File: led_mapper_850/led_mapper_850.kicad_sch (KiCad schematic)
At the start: 1082 parts, among them J1 Conn_02x12_Top_Bottom

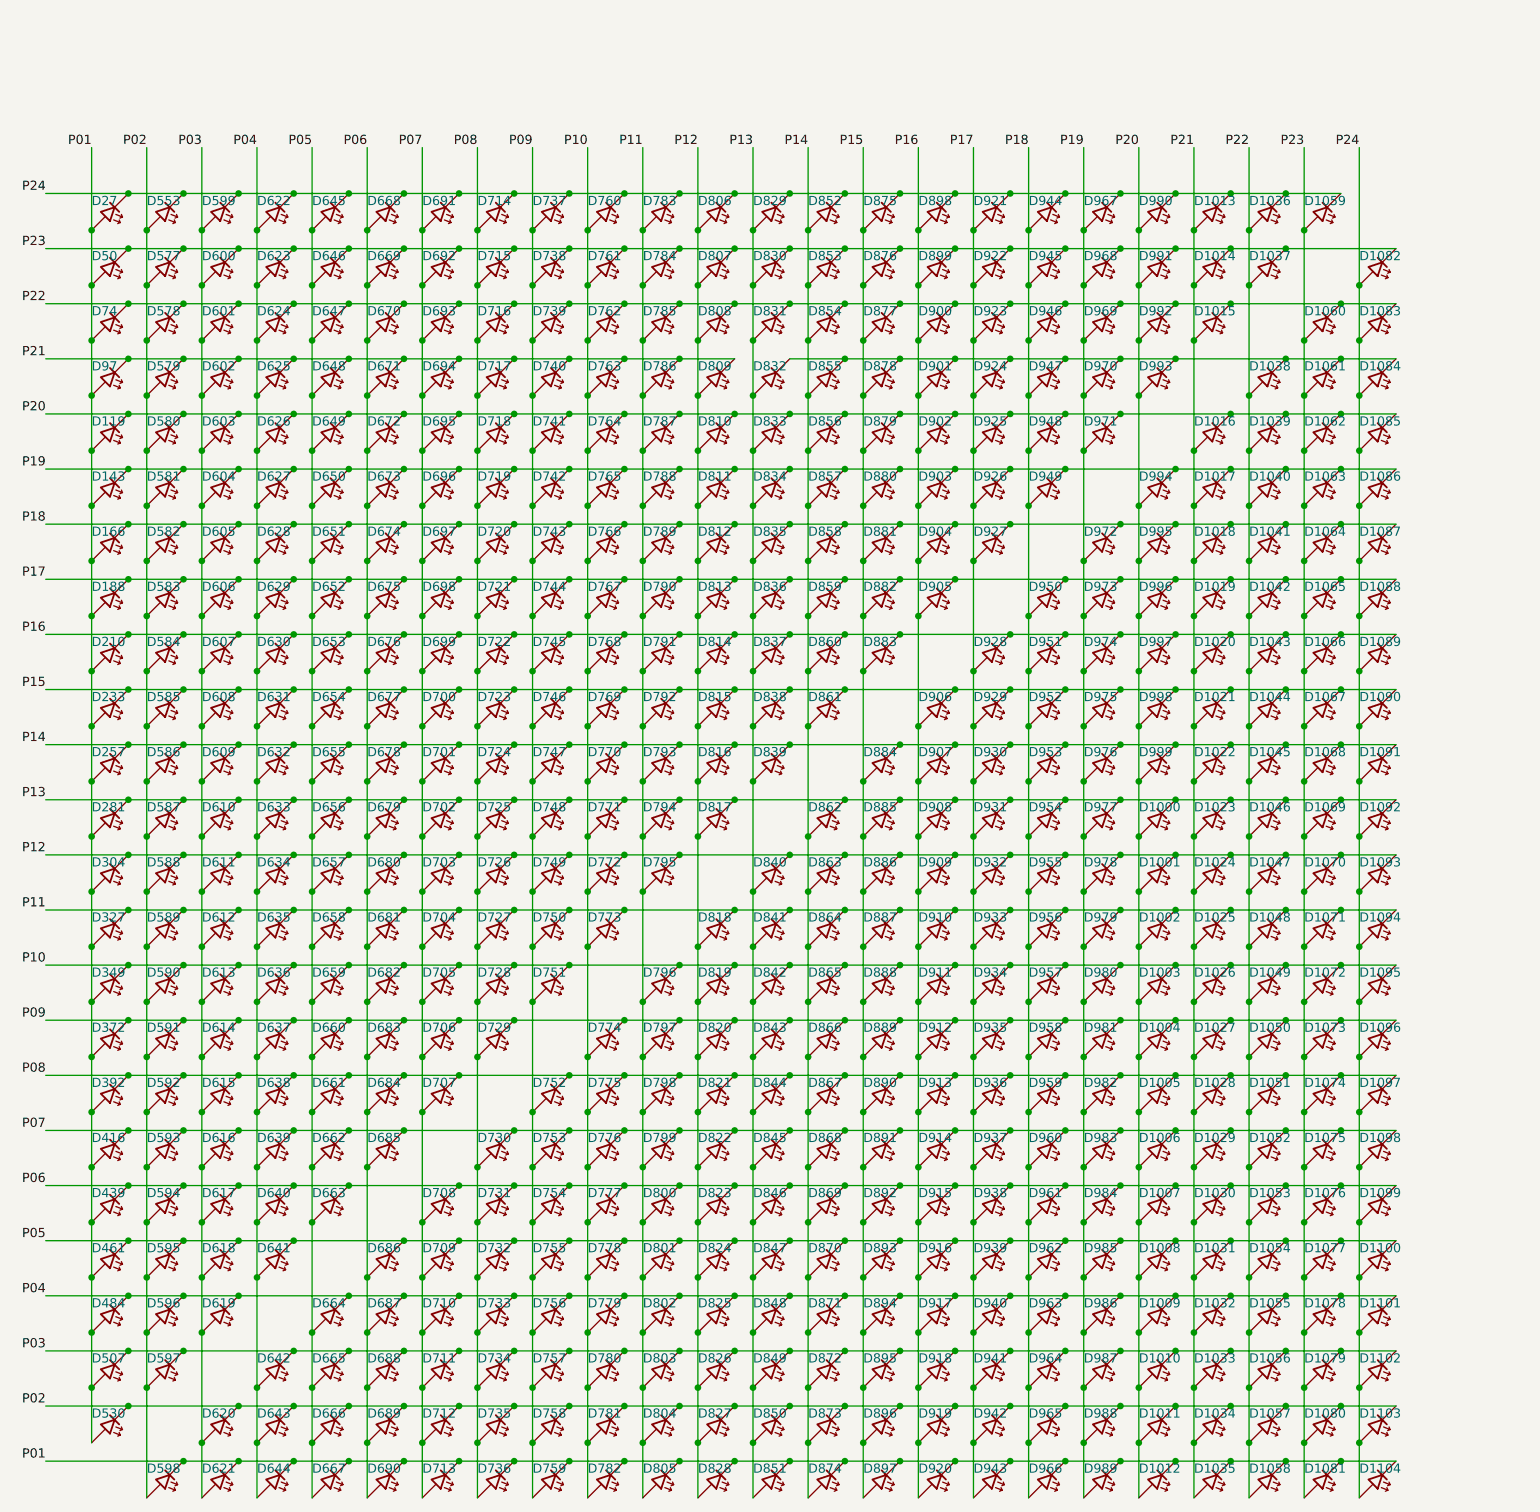
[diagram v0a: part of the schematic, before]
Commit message: remove old file
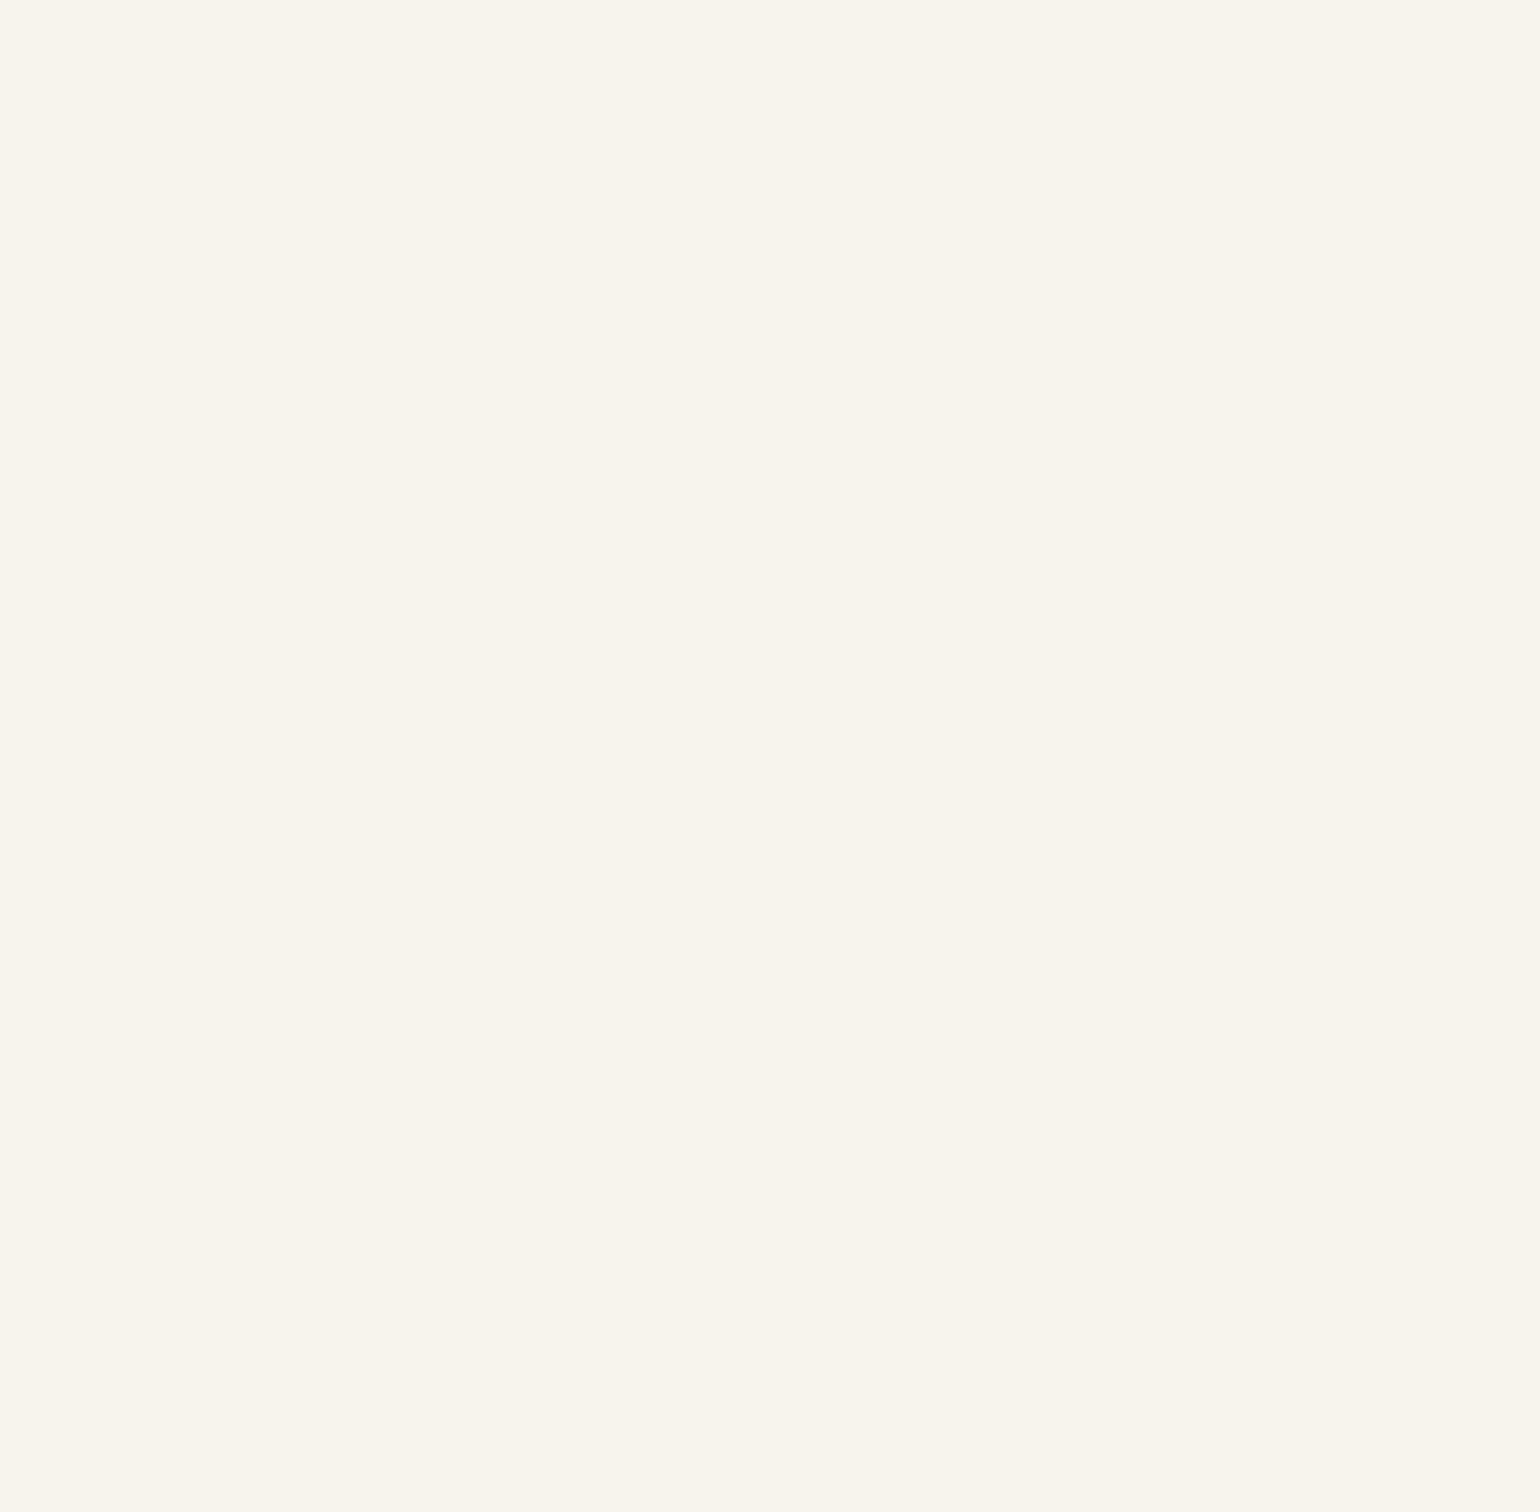
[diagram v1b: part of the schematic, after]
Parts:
- removed D1000, D1001, D1002, D1003, D1004, D1005, D1006, D1007, D1008, D1009, D1010, D1011, D1012, D1013, D1014, D1015, D1016, D1017, D1018, D1019, D1020, D1021, D1022, D1023, D1024, D1025, D1026, D1027, D1028, D1029, D1030, D1031, D1032, D1033, D1034, D1035, D1036, D1037, D1038, D1039, D1040, D1041, D1042, D1043, D1044, D1045, D1046, D1047, D1048, D1049, D1050, D1051, D1052, D1053, D1054, D1055, D1056, D1057, D1058, D1059, D1060, D1061, D1062, D1063, D1064, D1065, D1066, D1067, D1068, D1069, D1070, D1071, D1072, D1073, D1074, D1075, D1076, D1077, D1078, D1079, D1080, D1081, D1082, D1083, D1084, D1085, D1086, D1087, D1088, D1089, D1090, D1091, D1092, D1093, D1094, D1095, D1096, D1097, D1098, D1099, D1100, D1101, D1102, D1103, D1104, D119, D143, D166, D188, D210, D233, D257, D27, D281, D304, D327, D349, D372, D392, D416, D439, D461, D484, D50, D507, D530, D553, D577, D578, D579, D580, D581, D582, D583, D584, D585, D586, D587, D588, D589, D590, D591, D592, D593, D594, D595, D596, D597, D598, D599, D600, D601, D602, D603, D604, D605, D606, D607, D608, D609, D610, D611, D612, D613, D614, D615, D616, D617, D618, D619, D620, D621, D622, D623, D624, D625, D626, D627, D628, D629, D630, D631, D632, D633, D634, D635, D636, D637, D638, D639, D640, D641, D642, D643, D644, D645, D646, D647, D648, D649, D650, D651, D652, D653, D654, D655, D656, D657, D658, D659, D660, D661, D662, D663, D664, D665, D666, D667, D668, D669, D670, D671, D672, D673, D674, D675, D676, D677, D678, D679, D680, D681, D682, D683, D684, D685, D686, D687, D688, D689, D690, D691, D692, D693, D694, D695, D696, D697, D698, D699, D700, D701, D702, D703, D704, D705, D706, D707, D708, D709, D710, D711, D712, D713, D714, D715, D716, D717, D718, D719, D720, D721, D722, D723, D724, D725, D726, D727, D728, D729, D730, D731, D732, D733, D734, D735, D736, D737, D738, D739, D74, D740, D741, D742, D743, D744, D745, D746, D747, D748, D749, D750, D751, D752, D753, D754, D755, D756, D757, D758, D759, D760, D761, D762, D763, D764, D765, D766, D767, D768, D769, D770, D771, D772, D773, D774, D775, D776, D777, D778, D779, D780, D781, D782, D783, D784, D785, D786, D787, D788, D789, D790, D791, D792, D793, D794, D795, D796, D797, D798, D799, D800, D801, D802, D803, D804, D805, D806, D807, D808, D809, D810, D811, D812, D813, D814, D815, D816, D817, D818, D819, D820, D821, D822, D823, D824, D825, D826, D827, D828, D829, D830, D831, D832, D833, D834, D835, D836, D837, D838, D839, D840, D841, D842, D843, D844, D845, D846, D847, D848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: LED, LED_SMD:LED_0201_0603Metric, symbol Device:LED_45deg
